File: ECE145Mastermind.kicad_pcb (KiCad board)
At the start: 4 copper layers, 150.4 x 100.6 mm, 107 parts, among them J1 Conn_01x02_Socket, J10 Conn_01x01_Socket, J11 Conn_01x01_Socket, J12 Conn_01x01_Socket, J13 Conn_01x01_Socket, J14 Conn_01x01_Socket, J15 Conn_01x01_Socket, J16 Conn_01x01_Socket, J17 Conn_01x01_Socket, J2 Conn_01x01_Socket, J3 Conn_01x01_Socket, J4 Conn_01x01_Socket, J5 Conn_01x01_Socket, J6 Conn_01x01_Socket, J7 Conn_01x01_Socket, J8 Conn_01x01_Socket, J9 Conn_01x01_Socket, Q1 NMOS, SW1 SW_SPDT, SW2 SW_Push, U1 74LS08, U10 40106, U11 4053, U12 LM7805_TO220, U13 74LS194, U14 4053, U15 4051, U16 LM358, U17 LM324, U18 LM324, U19 74LS08, U2 74HCT00, U20 LM555xN, U21 74LS161, U22 74HCT00, U23 74HCT74, U24 74HCT00, U3 74LS73, U4 74LS194, U5 74LS148, U6 74LS73, U7 74LS194, U8 74LS139, U9 74HCT04

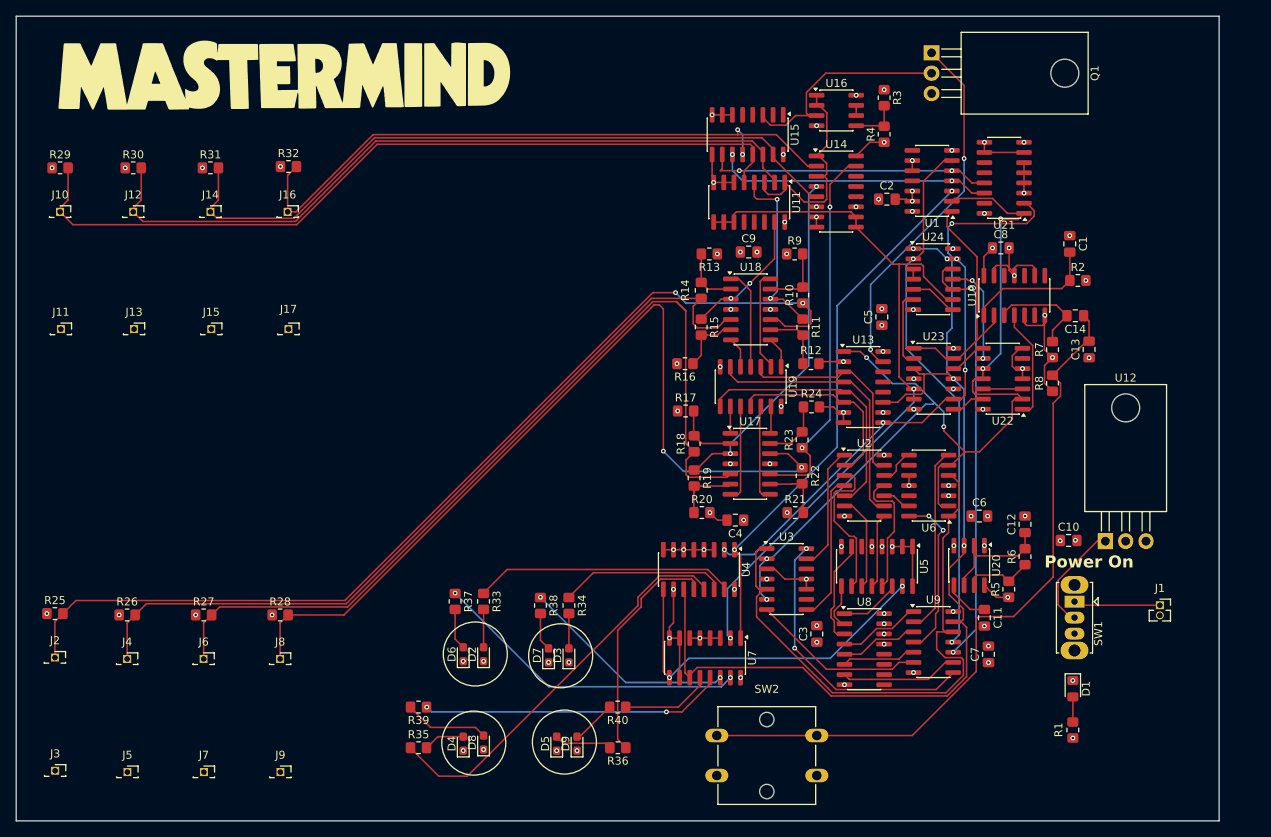
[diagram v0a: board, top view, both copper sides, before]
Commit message: Finished?
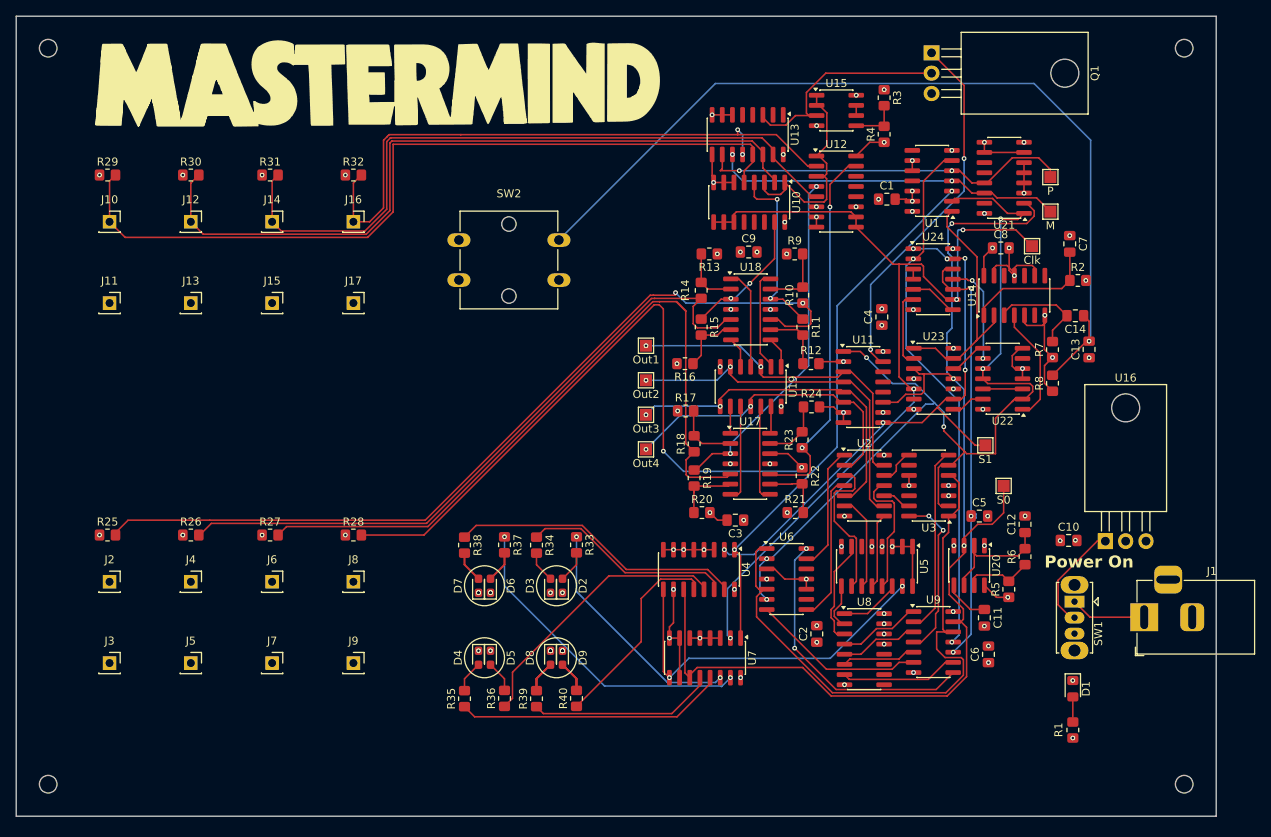
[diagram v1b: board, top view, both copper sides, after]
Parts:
- added REF**: MountingHole_2.2mm_M2, MountingHole:MountingHole_2.2mm_M2, F.Cu at (190.6, 42.3)
- added REF**: MountingHole_2.2mm_M2, MountingHole:MountingHole_2.2mm_M2, F.Cu at (190.6, 134.3)
- added REF**: MountingHole_2.2mm_M2, MountingHole:MountingHole_2.2mm_M2, F.Cu at (48.6, 42.3)
- added REF**: MountingHole_2.2mm_M2, MountingHole:MountingHole_2.2mm_M2, F.Cu at (48.6, 134.3)
- added TP1: Out1, TestPoint:TestPoint_Pad_1.5x1.5mm, F.Cu at (123.3, 79.5)
- added TP2: Out2, TestPoint:TestPoint_Pad_1.5x1.5mm, F.Cu at (123.3, 83.8)
- added TP3: Out3, TestPoint:TestPoint_Pad_1.5x1.5mm, F.Cu at (123.3, 88.1)
- added TP4: Out4, TestPoint:TestPoint_Pad_1.5x1.5mm, F.Cu at (123.3, 92.4)
- added TP5: S0, TestPoint:TestPoint_Pad_1.5x1.5mm, F.Cu at (168.0, 97.0)
- added TP6: S1, TestPoint:TestPoint_Pad_1.5x1.5mm, F.Cu at (165.8, 91.9)
- added TP7: Clk, TestPoint:TestPoint_Pad_1.5x1.5mm, F.Cu at (171.6, 67.0)
- added TP8: M, TestPoint:TestPoint_Pad_1.5x1.5mm, F.Cu at (173.9, 62.7)
- added TP9: P, TestPoint:TestPoint_Pad_1.5x1.5mm, F.Cu at (173.9, 58.4)
- D2, D4, D6, D8: value LED -> White LED
- D3, D5, D7, D9: value LED -> Red LED
- J1: footprint Connector_PinSocket_1.27mm:PinSocket_1x02_P1.27mm_Vertical -> Connector_BarrelJack:BarrelJack_Horizontal
- J10, J11, J12, J13, J14, J15, J16, J17, J2, J3, J4, J5, J6, J7, J8, J9: footprint Connector_PinSocket_1.27mm:PinSocket_1x01_P1.27mm_Vertical -> Connector_PinSocket_2.54mm:PinSocket_1x01_P2.54mm_Vertical
- R10, R14, R18, R22: value 2.2k -> 10k
- R33, R35: value 1k -> 2.2k
- R38, R40: value 2.2k -> 1k
- moved SW2 69.8 mm to (100.0, 66.2)
- moved J9 16.4 mm to (86.8, 119.1)
- moved J7 16.1 mm to (76.6, 119.1)
- moved J5 15.8 mm to (66.4, 119.1)
- moved R36 15.5 mm to (105.7, 123.5), turned to 90 degrees
- moved J3 15.1 mm to (56.3, 119.1)
- moved R39 14.8 mm to (109.7, 123.6), turned to 90 degrees
- moved R33 13.6 mm to (114.7, 104.4)
- moved D5 13.6 mm to (103.9, 118.5), turned to -90 degrees
- moved R28 13.6 mm to (86.8, 103.1)
- moved D8 13.5 mm to (111.4, 118.5), turned to -90 degrees
- moved J8 13.3 mm to (86.8, 109.0)
- moved D2 13.1 mm to (112.9, 109.5)
- moved R27 13.0 mm to (76.4, 103.1)
- moved J6 12.9 mm to (76.6, 109.0)
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- renumbered C2 to C1, C3 to C2, C4 to C3, C5 to C4, C6 to C5, C7 to C6, C1 to C7, U11 to U10, U13 to U11, U14 to U12, U15 to U13, U10 to U14, U16 to U15, U12 to U16, U6 to U3, U3 to U6
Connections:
- net /Misplaced LED/M1 renamed /M1
- net /Perfect LED/P2 renamed /P2
- R33 pad 1: /Perfect LED/P1 -> /M2
- R35 pad 1: /Perfect LED/P3 -> /M3
- R36 pad 1: /Perfect LED/P4 -> /P3
- R38 pad 1: /Misplaced LED/M2 -> /P1
- R39 pad 1: /Misplaced LED/M3 -> /M4
- R40 pad 1: /Misplaced LED/M4 -> /P4
- U4 pad 12: /Perfect LED/P4 -> /P4
- U4 pad 13: /Perfect LED/P3 -> /P3
- U4 pad 15: /Perfect LED/P1 -> /P1
- U7 pad 12: /Misplaced LED/M4 -> /M4
- U7 pad 13: /Misplaced LED/M3 -> /M3
- U7 pad 14: /Misplaced LED/M2 -> /M2
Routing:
- net /Perfect LED/P3: track 50.1 -> 0.00 mm
- net /Misplaced LED/M3: track 37.9 -> 0.00 mm, vias 2 -> 0
- net /P1: track 0.00 -> 36.6 mm
- net /P3: track 0.00 -> 34.5 mm
- net /M3: track 0.00 -> 33.7 mm
- net /Perfect LED/P1: track 32.6 -> 0.00 mm
- net /M2: track 0.00 -> 29.8 mm, vias 0 -> 2
- net /Perfect LED/P4: track 29.0 -> 0.00 mm
- net /Misplaced LED/M2: track 27.1 -> 0.00 mm, vias 2 -> 0
- net /P4: track 0.00 -> 25.5 mm
- net /M4: track 0.00 -> 23.2 mm
- net Net-(C13-Pad2): track 89.9 -> 112.5 mm, vias 0 -> 1
- net /C4: track 110.2 -> 91.0 mm
- net /M: track 94.5 -> 113.4 mm, vias 2 -> 4
- net /C3: track 110.7 -> 92.3 mm
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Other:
- board size 150.4 x 100.6 mm -> 150 x 100 mm
